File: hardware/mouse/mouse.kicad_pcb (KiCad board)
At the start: 4 copper layers, 44 x 68 mm, 82 parts, among them J2 JSTPH, J3 USB_C_Receptacle_USB2.0_14P, SW1 SW_SPST, SW2 SW_SPST, SW3 SW_SPST, SW4 SW_SPST, SW5 SW_SPST, SW6 SW_SPST, SW7 SW_SPST, SW8 RotaryEncoder, SW9 SW_SPST, U2 SPX3819M5-L-3-3, U3 MCP73831-2-OT, U4 TLV70019_SOT23-5, U5 nRF52840, U6 SPX3819M5-L-5-0, Y1 32.768 Hz, Y2 32 Hz

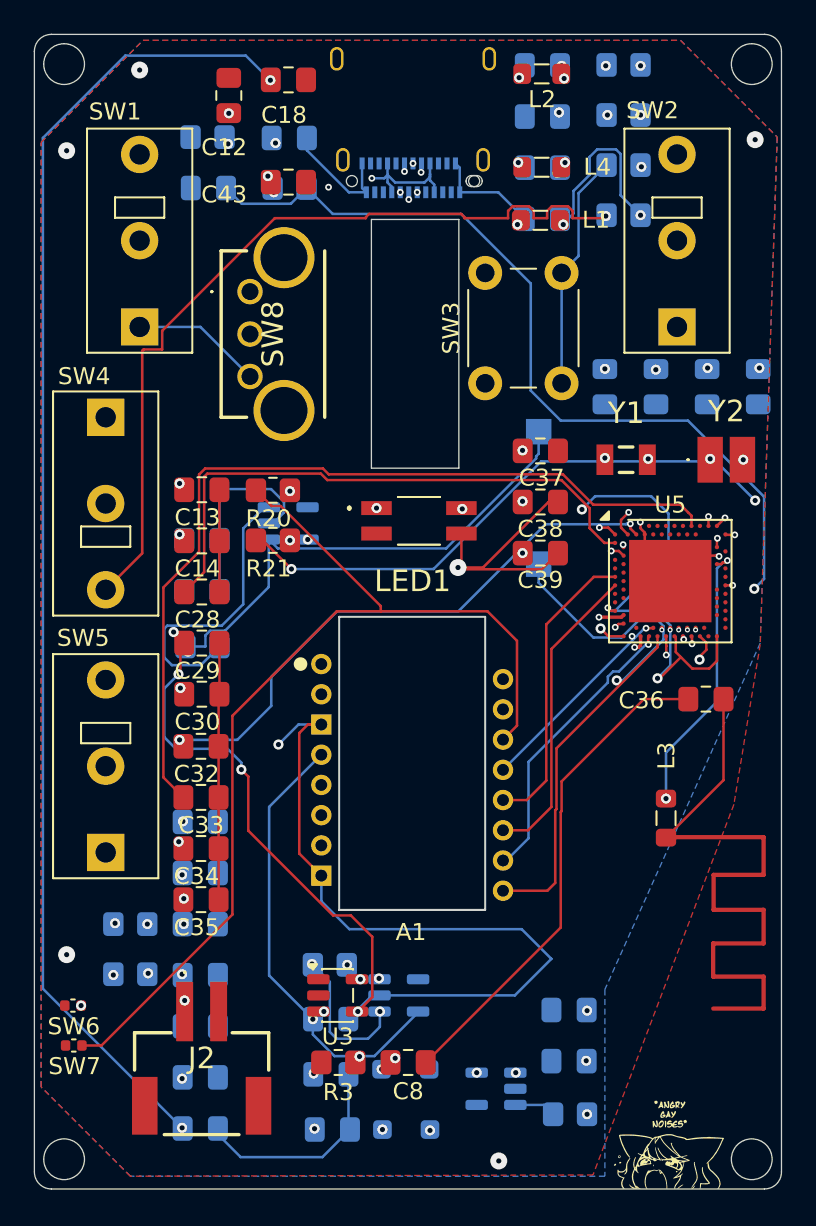
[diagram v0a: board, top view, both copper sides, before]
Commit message: meow :3
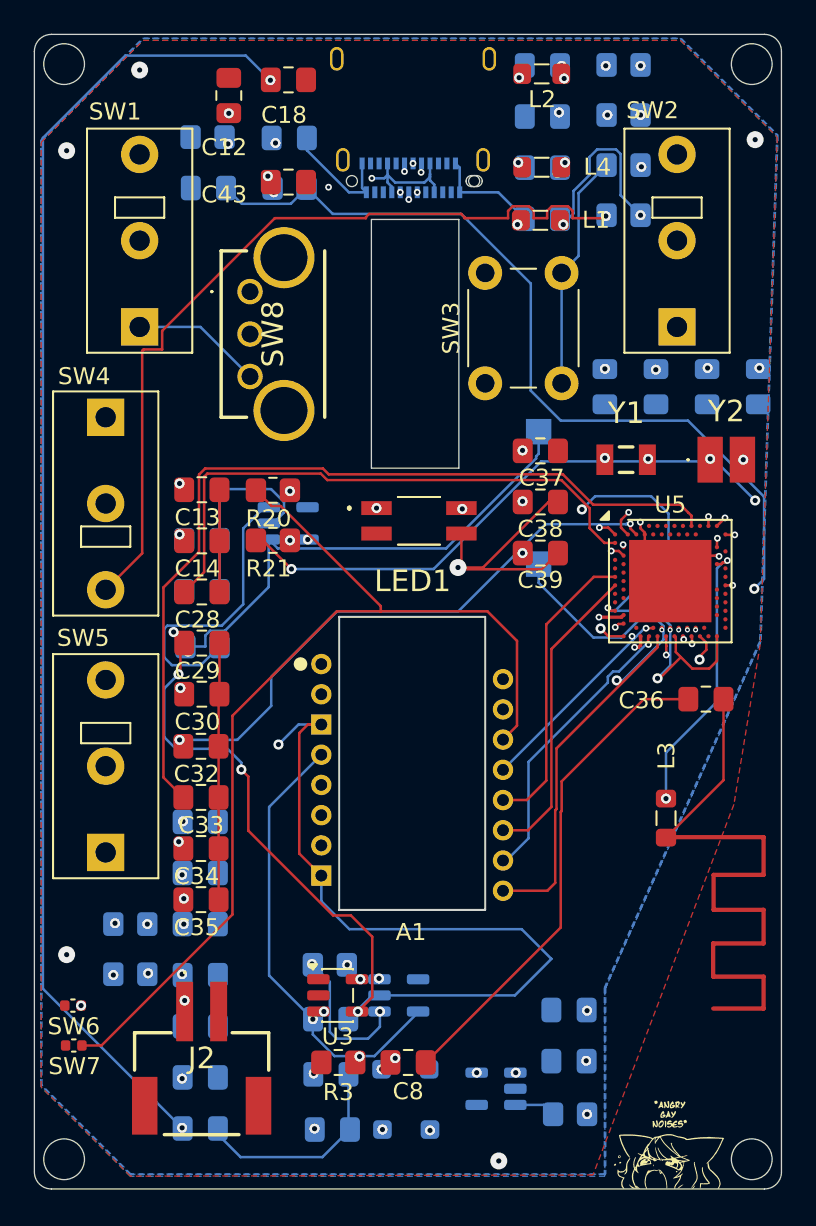
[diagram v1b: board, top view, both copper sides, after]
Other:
- copper layers 4 -> 6
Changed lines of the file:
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@@
 		(4 "In1.Cu" signal)
 		(6 "In2.Cu" signal)
+		(8 "In3.Cu" signal)
+		(10 "In4.Cu" signal)
 		(2 "B.Cu" signal)
 		(9 "F.Adhes" user "F.Adhesive")
@@
 			(layer "dielectric 2"
 				(type "core")
-				(thickness 1.24)
+				(thickness 0.535)
 				(material "FR4")
 				(epsilon_r 4.5)
@@
 				(loss_tangent 0.02)
 			)
+			(layer "In3.Cu"
+				(type "copper")
+				(thickness 0.035)
+			)
+			(layer "dielectric 4"
+				(type "core")
+				(thickness 0.535)
+				(material "FR4")
+				(epsilon_r 4.5)
+				(loss_tangent 0.02)
+			)
+			(layer "In4.Cu"
+				(type "copper")
+				(thickness 0.035)
+			)
+			(layer "dielectric 5"
+				(type "prepreg")
+				(thickness 0.1)
+				(material "FR4")
+				(epsilon_r 4.5)
+				(loss_tangent 0.02)
+			)
 			(layer "B.Cu"
 				(type "copper")
@@
 		(polygon
 			(pts
+				(xy 110.552305 74.783387) (xy 142.202305 74.783387) (xy 147.902305 80.483387) (xy 146.902305 110.283387)
+				(xy 137.752305 130.683387) (xy 137.752305 141.683387) (xy 109.802305 141.683387) (xy 104.552305 136.433387)
+				(xy 104.552305 80.783387)
+			)
+		)
+	)
+	(zone
+		(net 9)
+		(net_name "GND")
+		(layer "B.Cu")
+		(hatch edge 0.5)
+		(connect_pads
+			(clearance 0.5)
+		)
+		(min_thickness 0.25)
+		(filled_areas_thickness no)
+		(fill yes
+			(thermal_gap 0.5)
+			(thermal_bridge_width 0.5)
+		)
+		(polygon
+			(pts
 				(xy 110.5 74.9) (xy 142.15 74.9) (xy 147.85 80.6) (xy 146.85 110.4) (xy 137.7 130.8) (xy 137.7 141.8)
 				(xy 109.75 141.8) (xy 104.5 136.55) (xy 104.5 80.9)
 			)
 		)
+	)
+	(zone
+		(net 9)
+		(net_name "GND")
+		(layer "B.Cu")
+		(hatch edge 0.5)
+		(connect_pads
+			(clearance 0.5)
+		)
+		(min_thickness 0.25)
+		(filled_areas_thickness no)
+		(fill yes
+			(thermal_gap 0.5)
+			(thermal_bridge_width 0.5)
+		)
+		(polygon
+			(pts
+				(xy 110.468318 74.779652) (xy 142.118318 74.779652) (xy 147.818318 80.479652) (xy 146.818318 110.279652)
+				(xy 137.668318 130.679652) (xy 137.668318 141.679652) (xy 109.718318 141.679652) (xy 104.468318 136.429652)
+				(xy 104.468318 80.779652)
+			)
+		)
